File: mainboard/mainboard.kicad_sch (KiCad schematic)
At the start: 29 parts, among them J1 USB_C_Receptacle_USB2.0_16P, SW1 SW_SPST, SW2 SW_SPST, U1 AMS1117-3.3, U2 ESP32-S3-WROOM-1, U3 TCA9548ARGER, U4 ADXL345, U5 ADXL375

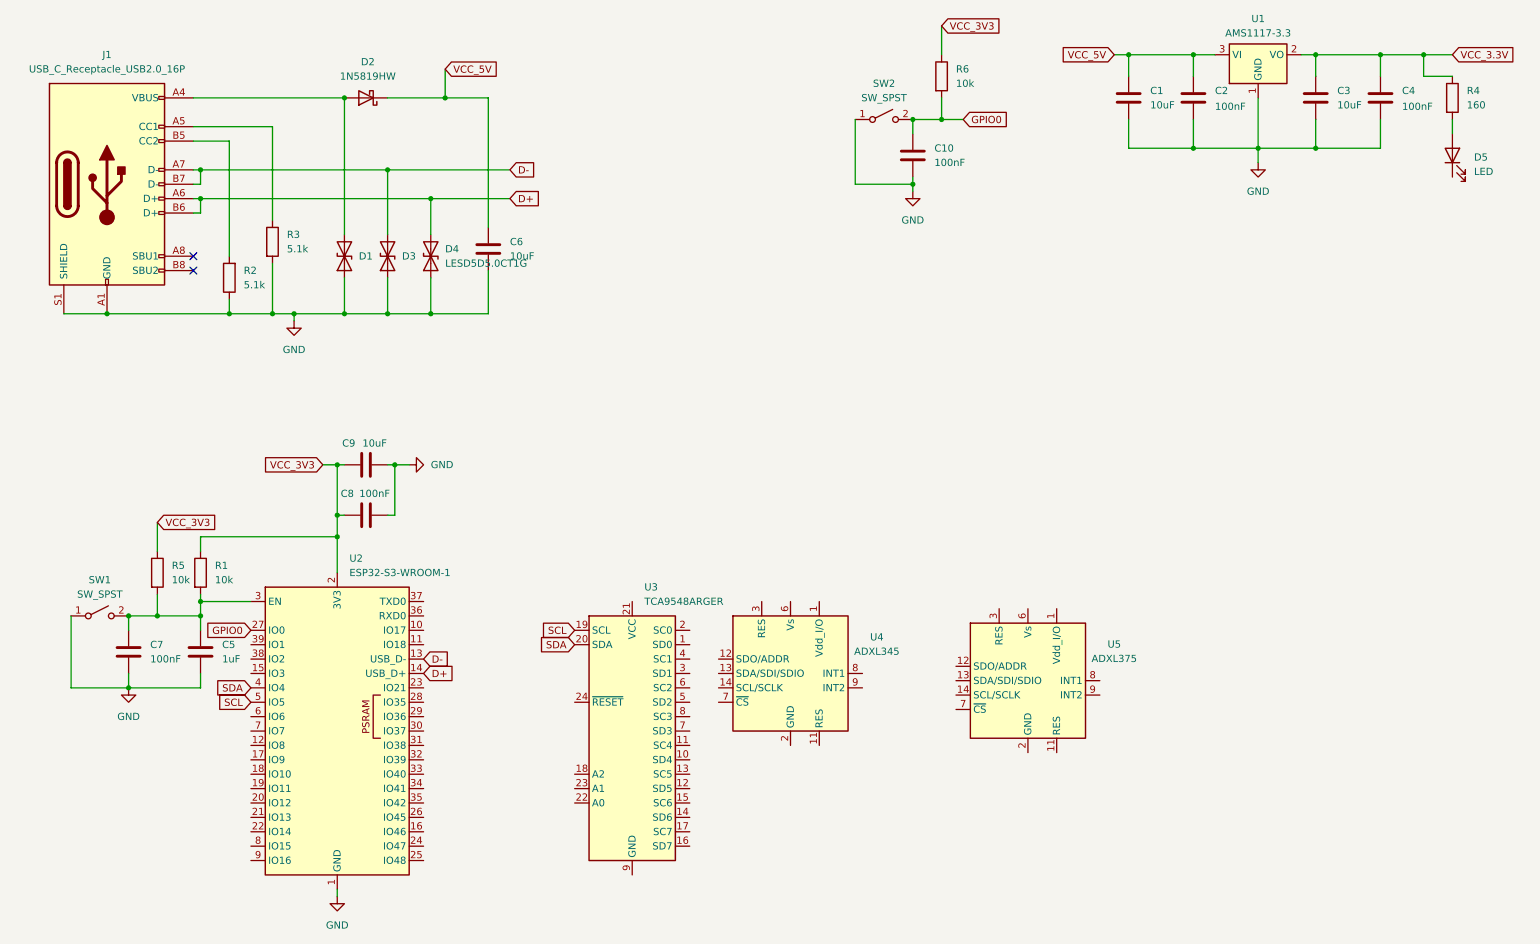
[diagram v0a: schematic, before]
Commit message: updated mainboard
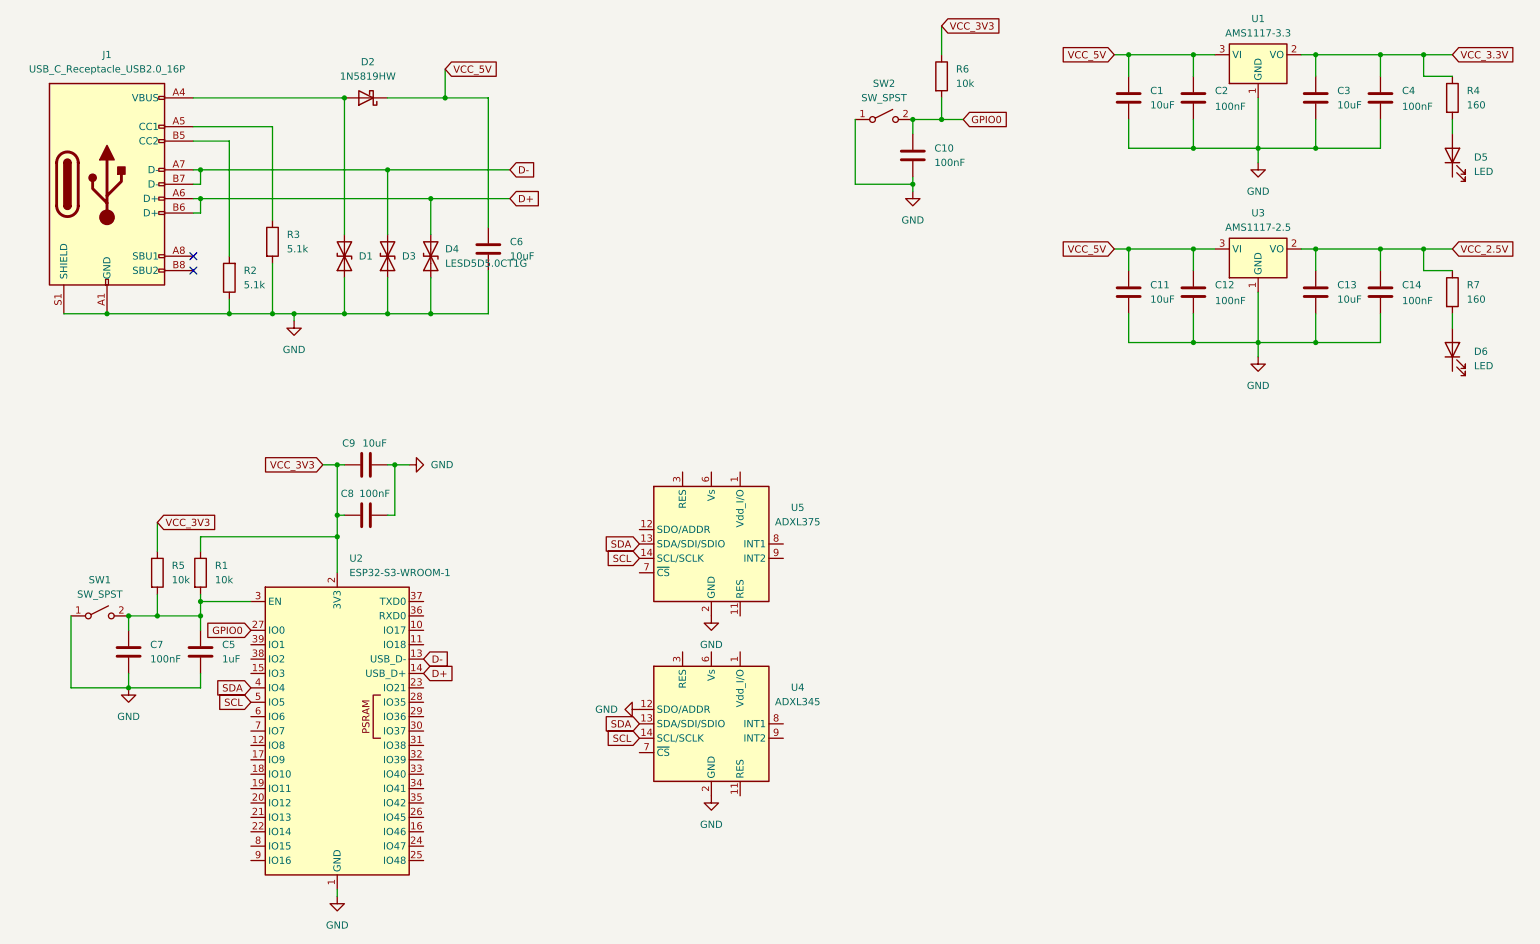
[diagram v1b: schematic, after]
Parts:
- removed U3: TCA9548ARGER, Package_DFN_QFN:Texas_RGE0024C_VQFN-24-1EP_4x4mm_P0.5mm_EP2.1x2.1mm, symbol Interface_Expansion:TCA9548ARGER
- added C11, C13: 10uF, Capacitor_SMD:C_0805_2012Metric, symbol Device:C
- added C12, C14: 100nF, Capacitor_SMD:C_0603_1608Metric, symbol Device:C
- added D6: LED, LED_SMD:LED_0805_2012Metric, symbol Device:LED
- added R7: 160, Resistor_SMD:R_0603_1608Metric, symbol Device:R
- added U3: AMS1117-2.5, Package_TO_SOT_SMD:SOT-223-3_TabPin2, symbol Regulator_Linear:AMS1117-2.5
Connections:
- net GND: now also U4.12 (SDO/ADDR), U4.2 (GND), U4.4 (GND), U4.5 (GND), U5.2 (GND), U5.4 (GND), U5.5 (GND), C11.2, C12.2, C13.2, C14.2, U3.1 (GND)
- net SCL: now also U4.14 (SCL/SCLK), U5.14 (SCL/SCLK)
- net SDA: now also U4.13 (SDA/SDI/SDIO), U5.13 (SDA/SDI/SDIO)
- net VCC_5V: now also C11.1, C12.1, U3.3 (VI)
- new net: D6.2 (A), R7.2
- new net VCC_2.5V: C13.1, C14.1, R7.1, U3.2 (VO)
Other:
- moved on the sheet: U4, U5
